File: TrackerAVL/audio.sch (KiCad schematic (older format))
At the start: 35 parts, among them U401 NAU8814

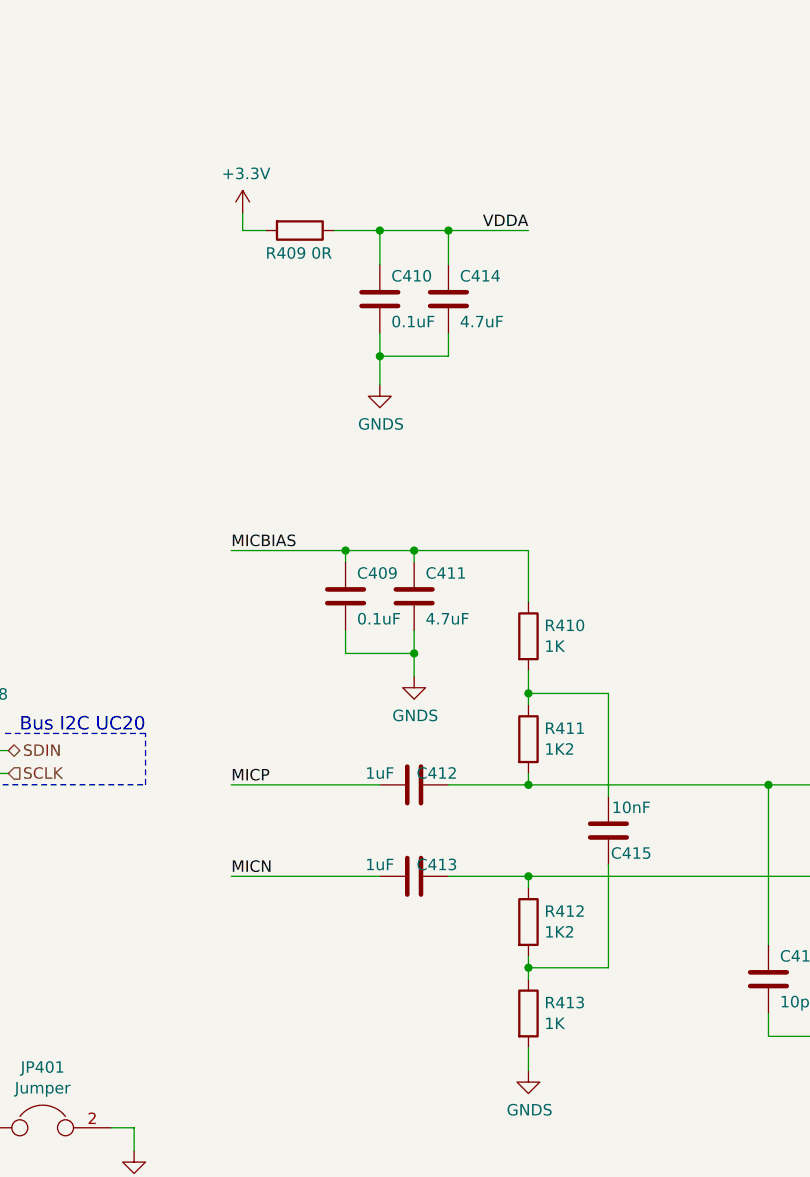
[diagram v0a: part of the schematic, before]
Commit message: Cambios en sch
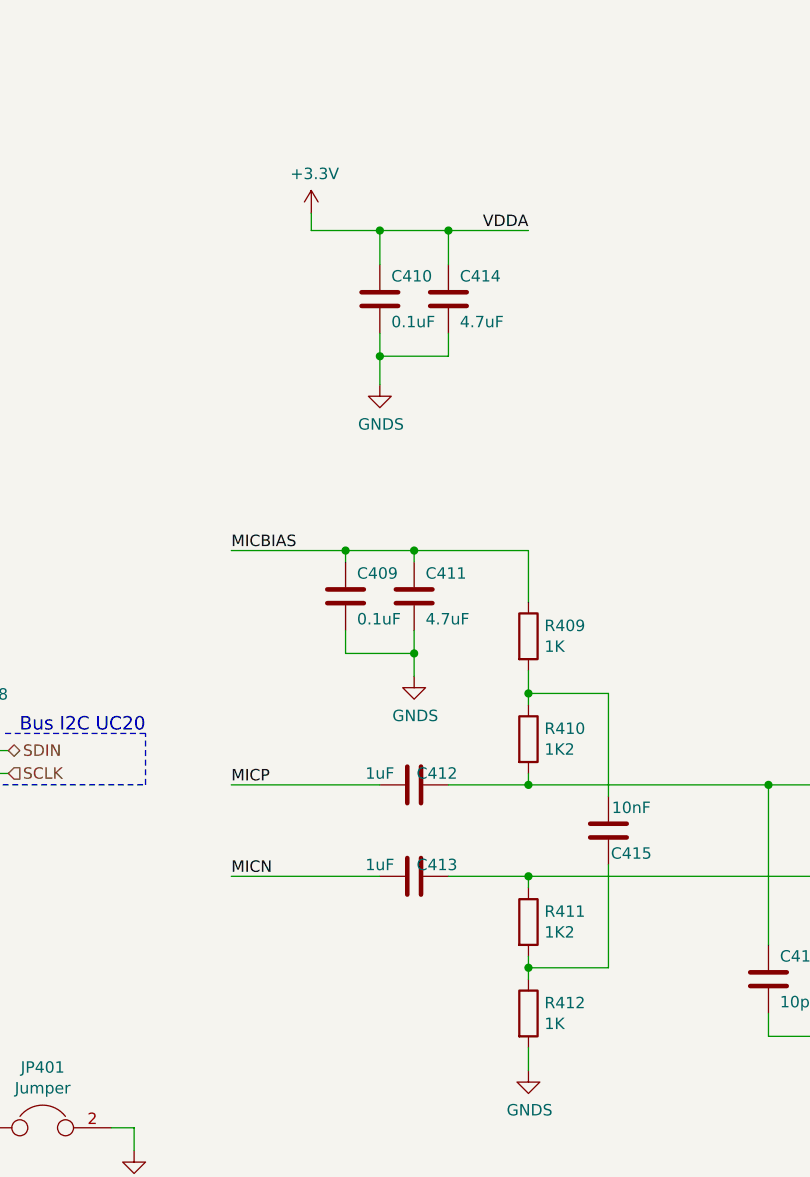
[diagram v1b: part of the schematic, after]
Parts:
- removed R409: 0R, symbol Device:R
- renumbered R410 to R409, R411 to R410, R412 to R411, R413 to R412
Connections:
- net VDDA is gone; now on net +3V3: C410.1, C414.1, U401.2 (VDDA)
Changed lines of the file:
@@
 	10325 4800 10325 4500
 $Comp
-L power:GND #PWR0418
+L power:GND #PWR0420
 U 1 1 5BCE86F7
 P 9925 5250
-F 0 "#PWR0418" H 9925 5000 50  0001 C CNN
+F 0 "#PWR0420" H 9925 5000 50  0001 C CNN
 F 1 "GND" H 9930 5077 50  0000 C CNN
 F 2 "" H 9925 5250 50  0001 C CNN
@@
 	7375 4500 7725 4500
 $Comp
-L Device:R R411
+L Device:R R410
 U 1 1 5BD28920
 P 7725 3900
-F 0 "R411" H 7795 3946 50  0000 L CNN
+F 0 "R410" H 7795 3946 50  0000 L CNN
 F 1 "1K2" H 7795 3855 50  0000 L CNN
 F 2 "" V 7655 3900 50  0001 C CNN
@@
 	7725 4050 7725 4100
 $Comp
-L Device:R R410
+L Device:R R409
 U 1 1 5BD2C760
 P 7725 3450
-F 0 "R410" H 7795 3496 50  0000 L CNN
+F 0 "R409" H 7795 3496 50  0000 L CNN
 F 1 "1K" H 7795 3405 50  0000 L CNN
 F 2 "" V 7655 3450 50  0001 C CNN
@@
 $EndComp
 $Comp
-L Device:R R412
+L Device:R R411
 U 1 1 5BD2C7B4
 P 7725 4700
-F 0 "R412" H 7795 4746 50  0000 L CNN
+F 0 "R411" H 7795 4746 50  0000 L CNN
 F 1 "1K2" H 7795 4655 50  0000 L CNN
 F 2 "" V 7655 4700 50  0001 C CNN
@@
 $EndComp
 $Comp
-L Device:R R413
+L Device:R R412
 U 1 1 5BD2C816
 P 7725 5100
-F 0 "R413" H 7795 5146 50  0000 L CNN
+F 0 "R412" H 7795 5146 50  0000 L CNN
 F 1 "1K" H 7795 5055 50  0000 L CNN
 F 2 "" V 7655 5100 50  0001 C CNN
@@
 $EndComp
 $Comp
-L power:GND #PWR0417
+L power:GND #PWR0419
 U 1 1 5BDB5E07
 P 9075 5250
-F 0 "#PWR0417" H 9075 5000 50  0001 C CNN
+F 0 "#PWR0419" H 9075 5000 50  0001 C CNN
 F 1 "GND" H 9080 5077 50  0000 C CNN
 F 2 "" H 9075 5250 50  0001 C CNN
@@
 Wire Wire Line
 	8775 4100 9075 4100
-$Comp
-L Device:R R409
-U 1 1 5BDCA93E
-P 6725 1675
-F 0 "R409" V 6825 1525 50  0000 L CNN
-F 1 "0R" V 6825 1725 50  0000 L CNN
-F 2 "" V 6655 1675 50  0001 C CNN
-F 3 "~" H 6725 1675 50  0001 C CNN
-	1    6725 1675
-	0    1    1    0
-$EndComp
-Wire Wire Line
-	6475 1600 6475 1675
-Wire Wire Line
-	6475 1675 6575 1675
+Wire Wire Line
+	6775 1600 6775 1675
 Text Label 2075 3650 0    50   ~ 0
 VDDA
 Wire Wire Line
 	2075 3650 2750 3650
-Wire Wire Line
-	6875 1675 7075 1675
 Wire Wire Line
 	7075 1675 7075 1825
@@
 Connection ~ 2400 4400
 $Comp
-L power:+3.3V #PWR0413
+L power:+3.3V #PWR0415
 U 1 1 5BE2A98A
-P 6475 1600
-F 0 "#PWR0413" H 6475 1450 50  0001 C CNN
-F 1 "+3.3V" H 6490 1773 50  0000 C CNN
-F 2 "" H 6475 1600 50  0001 C CNN
-F 3 "" H 6475 1600 50  0001 C CNN
-	1    6475 1600
+P 6775 1600
+F 0 "#PWR0415" H 6775 1450 50  0001 C CNN
+F 1 "+3.3V" H 6790 1773 50  0000 C CNN
+F 2 "" H 6775 1600 50  0001 C CNN
+F 3 "" H 6775 1600 50  0001 C CNN
+	1    6775 1600
 	1    0    0    -1
 $EndComp
@@
 $EndComp
 $Comp
-L power:GND #PWR0104
+L power:GND #PWR0413
 U 1 1 5C00FD89
 P 5200 5700
-F 0 "#PWR0104" H 5200 5450 50  0001 C CNN
+F 0 "#PWR0413" H 5200 5450 50  0001 C CNN
 F 1 "GND" H 5205 5527 50  0000 C CNN
 F 2 "" H 5200 5700 50  0001 C CNN
@@
 $EndComp
 $Comp
-L power:GNDS #PWR0105
+L power:GNDS #PWR0414
 U 1 1 5C020B55
 P 6000 5700
-F 0 "#PWR0105" H 6000 5450 50  0001 C CNN
+F 0 "#PWR0414" H 6000 5450 50  0001 C CNN
 F 1 "GNDS" H 6005 5527 50  0000 C CNN
 F 2 "" H 6000 5700 50  0001 C CNN
@@
 	6000 5600 6000 5700
 $Comp
-L power:GNDS #PWR0106
+L power:GNDS #PWR0405
 U 1 1 5C037CDB
 P 2550 3400
-F 0 "#PWR0106" H 2550 3150 50  0001 C CNN
+F 0 "#PWR0405" H 2550 3150 50  0001 C CNN
 F 1 "GNDS" V 2450 3350 50  0000 C CNN
 F 2 "" H 2550 3400 50  0001 C CNN
@@
 	3750 1900 3750 2050
 $Comp
-L power:GNDS #PWR0107
+L power:GNDS #PWR0409
 U 1 1 5C0A29B2
 P 4250 2550
-F 0 "#PWR0107" H 4250 2300 50  0001 C CNN
+F 0 "#PWR0409" H 4250 2300 50  0001 C CNN
 F 1 "GNDS" H 4255 2377 50  0000 C CNN
 F 2 "" H 4250 2550 50  0001 C CNN
@@
 Connection ~ 4250 2450
 $Comp
-L power:GNDS #PWR0108
+L power:GNDS #PWR0403
 U 1 1 5C0B3D39
 P 2075 3750
-F 0 "#PWR0108" H 2075 3500 50  0001 C CNN
+F 0 "#PWR0403" H 2075 3500 50  0001 C CNN
 F 1 "GNDS" V 2075 3525 50  0000 C CNN
 F 2 "" H 2075 3750 50  0001 C CNN
@@
 $EndComp
 $Comp
-L power:GNDS #PWR0109
+L power:GNDS #PWR0421
 U 1 1 5C0BF87B
 P 10325 5250
-F 0 "#PWR0109" H 10325 5000 50  0001 C CNN
+F 0 "#PWR0421" H 10325 5000 50  0001 C CNN
 F 1 "GNDS" H 10330 5077 50  0000 C CNN
 F 2 "" H 10325 5250 50  0001 C CNN
@@
 	10325 5250 10325 5100
 $Comp
-L power:GNDS #PWR0110
+L power:GNDS #PWR0418
 U 1 1 5C0D0AA1
 P 7725 5350
-F 0 "#PWR0110" H 7725 5100 50  0001 C CNN
+F 0 "#PWR0418" H 7725 5100 50  0001 C CNN
 F 1 "GNDS" H 7730 5177 50  0000 C CNN
 F 2 "" H 7725 5350 50  0001 C CNN
@@
 $EndComp
 $Comp
-L power:GNDS #PWR0111
+L power:GNDS #PWR0417
 U 1 1 5C0D67A2
 P 7225 3625
-F 0 "#PWR0111" H 7225 3375 50  0001 C CNN
+F 0 "#PWR0417" H 7225 3375 50  0001 C CNN
 F 1 "GNDS" H 7230 3452 50  0000 C CNN
 F 2 "" H 7225 3625 50  0001 C CNN
@@
 $EndComp
 $Comp
-L power:GNDS #PWR0112
+L power:GNDS #PWR0416
 U 1 1 5C0DC575
 P 7075 2350
-F 0 "#PWR0112" H 7075 2100 50  0001 C CNN
+F 0 "#PWR0416" H 7075 2100 50  0001 C CNN
 F 1 "GNDS" H 7080 2177 50  0000 C CNN
 F 2 "" H 7075 2350 50  0001 C CNN
@@
 $EndComp
 $Comp
-L power:GNDS #PWR0113
+L power:GNDS #PWR0410
 U 1 1 5C0E7FA4
 P 4550 3550
-F 0 "#PWR0113" H 4550 3300 50  0001 C CNN
+F 0 "#PWR0410" H 4550 3300 50  0001 C CNN
 F 1 "GNDS" V 4450 3500 50  0000 C CNN
 F 2 "" H 4550 3550 50  0001 C CNN
@@
 	7725 3600 7725 3700
 Connection ~ 7725 3700
+Wire Wire Line
+	6775 1675 7075 1675
 $EndSCHEMATC

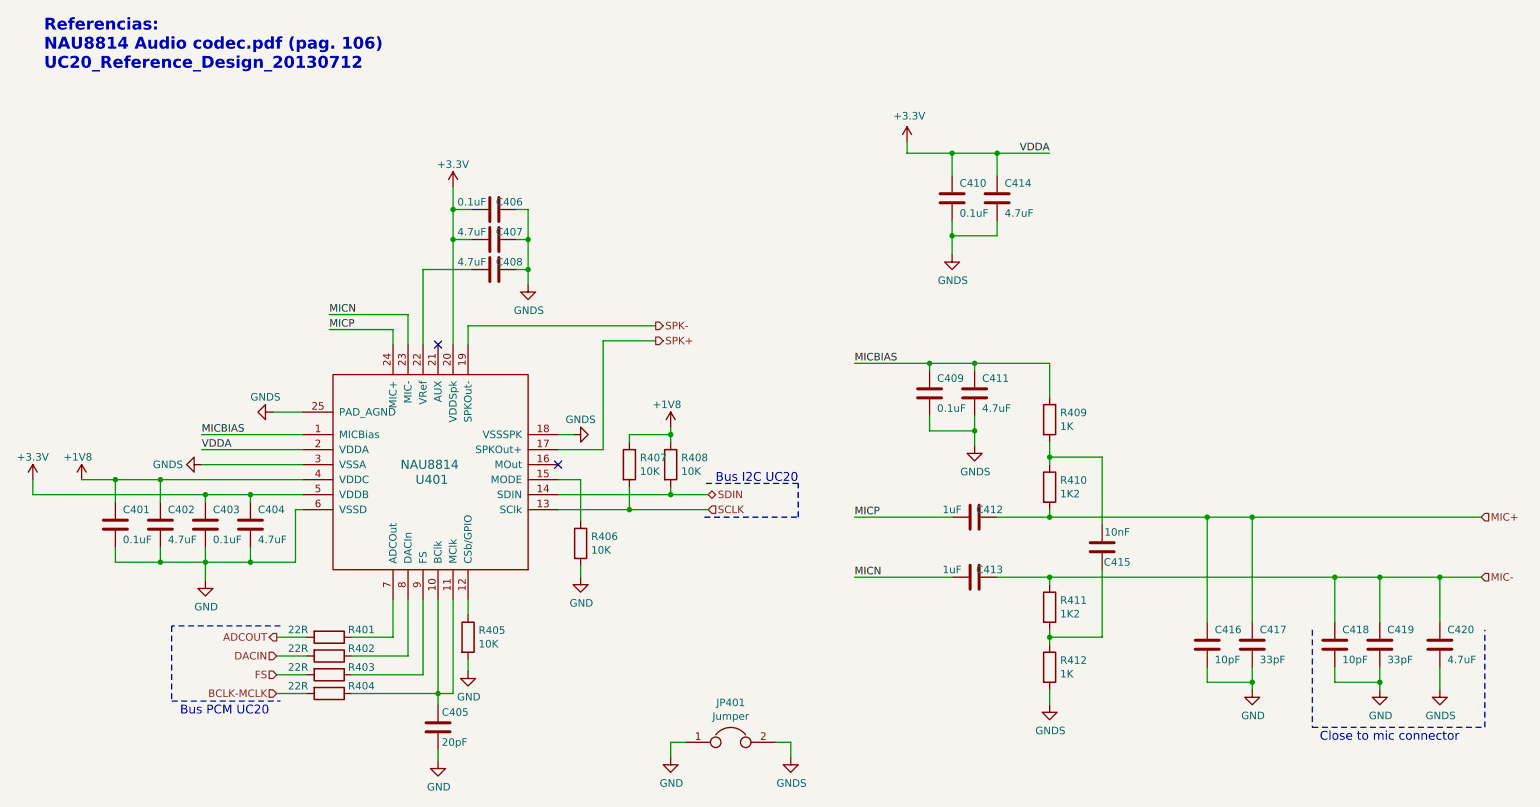
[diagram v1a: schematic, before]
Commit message: Cambios en sch
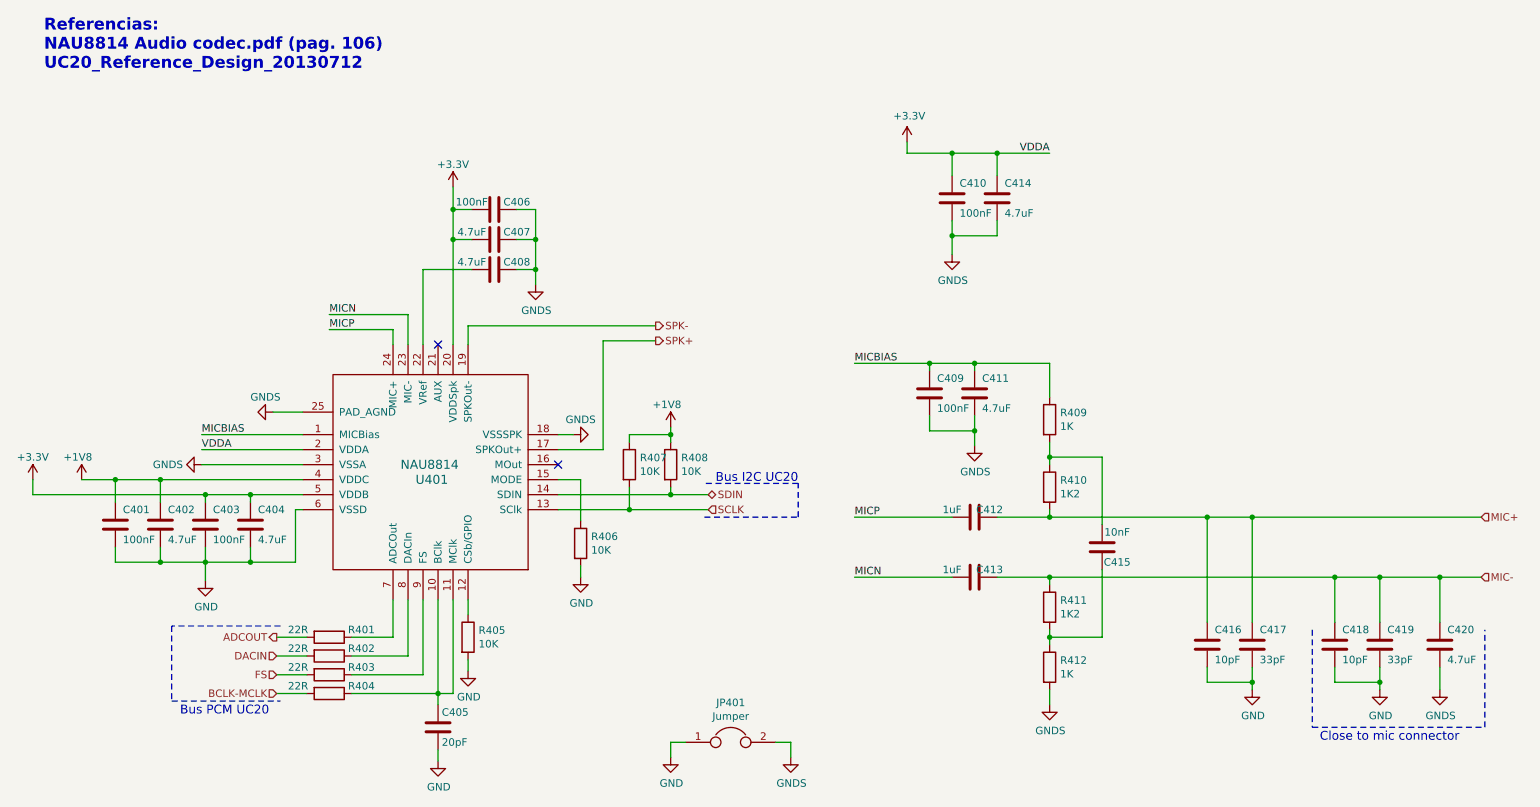
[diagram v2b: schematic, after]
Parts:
- C401, C403, C406, C409, C410: value 0.1uF -> 100nF; footprint (none) -> Capacitor_SMD:C_0805_2012Metric_Pad1.15x1.40mm_HandSolder
- C402, C404, C405, C407, C408, C411, C412, C413, C414, C415, C416, C417, C418, C419, C420: footprint (none) -> Capacitor_SMD:C_0805_2012Metric_Pad1.15x1.40mm_HandSolder
- JP401: footprint (none) -> Jumper:SolderJumper-2_P1.3mm_Bridged_Pad1.0x1.5mm
- R401, R402, R403, R404, R405, R406, R407, R408, R409, R410, R411, R412: footprint (none) -> Resistor_SMD:R_0805_2012Metric_Pad1.15x1.40mm_HandSolder

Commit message: Se modifica huella NAU8814 a QFN-24_HandSoldering
Falta modificar resto de huellas
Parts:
- U401: footprint nau8814:NAU8814_QFN-24_4x4mm_Pitch0.5mm_EPAD -> nau8814:NAU8814_QFN-24_4x4mm_Pitch0.5mm_EPAD_HandSoldering
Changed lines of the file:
@@
 F 0 "U401" H 3500 3750 60  0000 L CNN
 F 1 "NAU8814" H 3400 3850 60  0000 L CNN
-F 2 "nau8814:NAU8814_QFN-24_4x4mm_Pitch0.5mm_EPAD" H 3600 3800 60  0001 C CNN
+F 2 "nau8814:NAU8814_QFN-24_4x4mm_Pitch0.5mm_EPAD_HandSoldering" H 3600 3800 60  0001 C CNN
 F 3 "" H 3600 3800 60  0001 C CNN
 	1    3600 3800

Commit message: Pendiente revisión PCB y esquemático
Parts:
- U401: footprint nau8814:NAU8814_QFN-24_4x4mm_Pitch0.5mm_EPAD_HandSoldering -> nau8814:NAU8814_QFN-24_4x4mm_Pitch0.5mm_EPAD
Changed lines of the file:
@@
 F 0 "U401" H 3500 3750 60  0000 L CNN
 F 1 "NAU8814" H 3400 3850 60  0000 L CNN
-F 2 "nau8814:NAU8814_QFN-24_4x4mm_Pitch0.5mm_EPAD_HandSoldering" H 3600 3800 60  0001 C CNN
+F 2 "nau8814:NAU8814_QFN-24_4x4mm_Pitch0.5mm_EPAD" H 3600 3800 60  0001 C CNN
 F 3 "" H 3600 3800 60  0001 C CNN
 	1    3600 3800
